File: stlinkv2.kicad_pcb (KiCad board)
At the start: 2 copper layers, 54 parts, among them J1 TX, J2 RX, J3 JTAG, J4 SWIMM, J5 USB_B, U1 AZ1117-3.3, U2 STM32F103C8Tx, Y1 8M

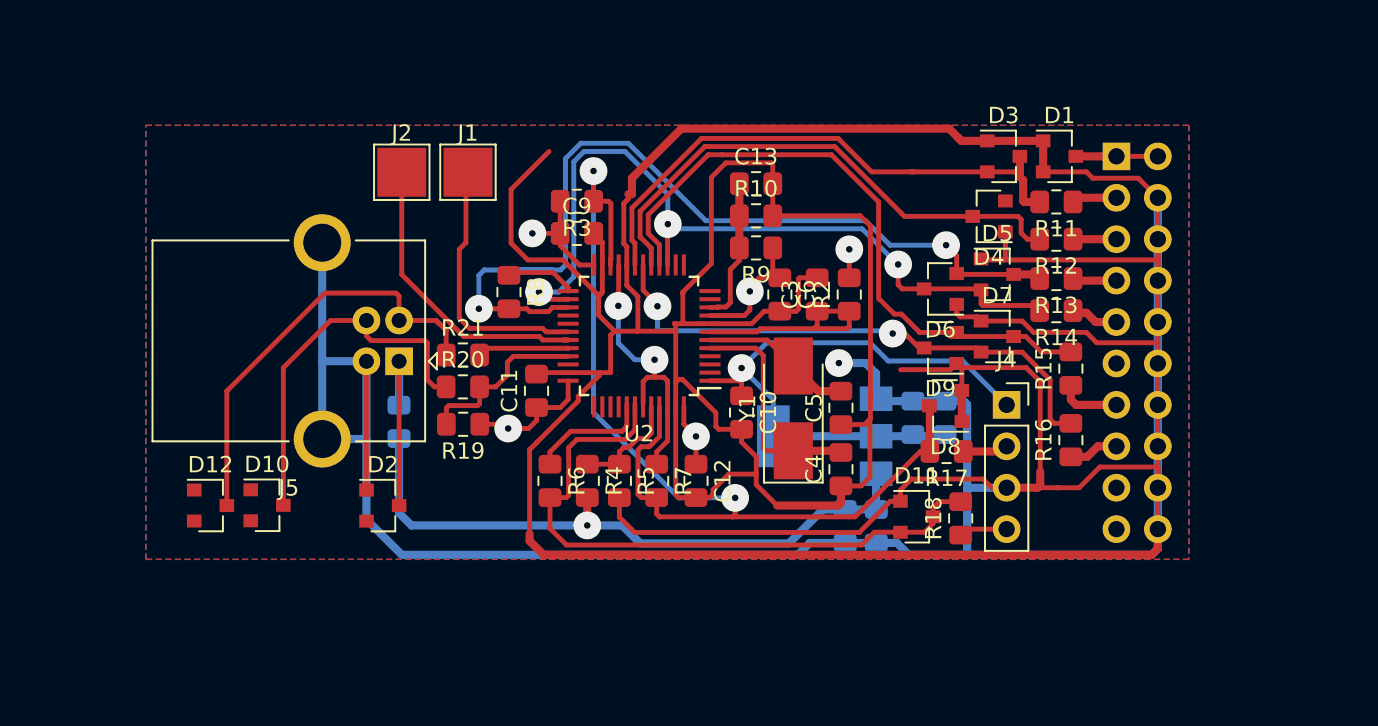
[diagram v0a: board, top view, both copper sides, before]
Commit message: добавил светодиоды, проверю без них
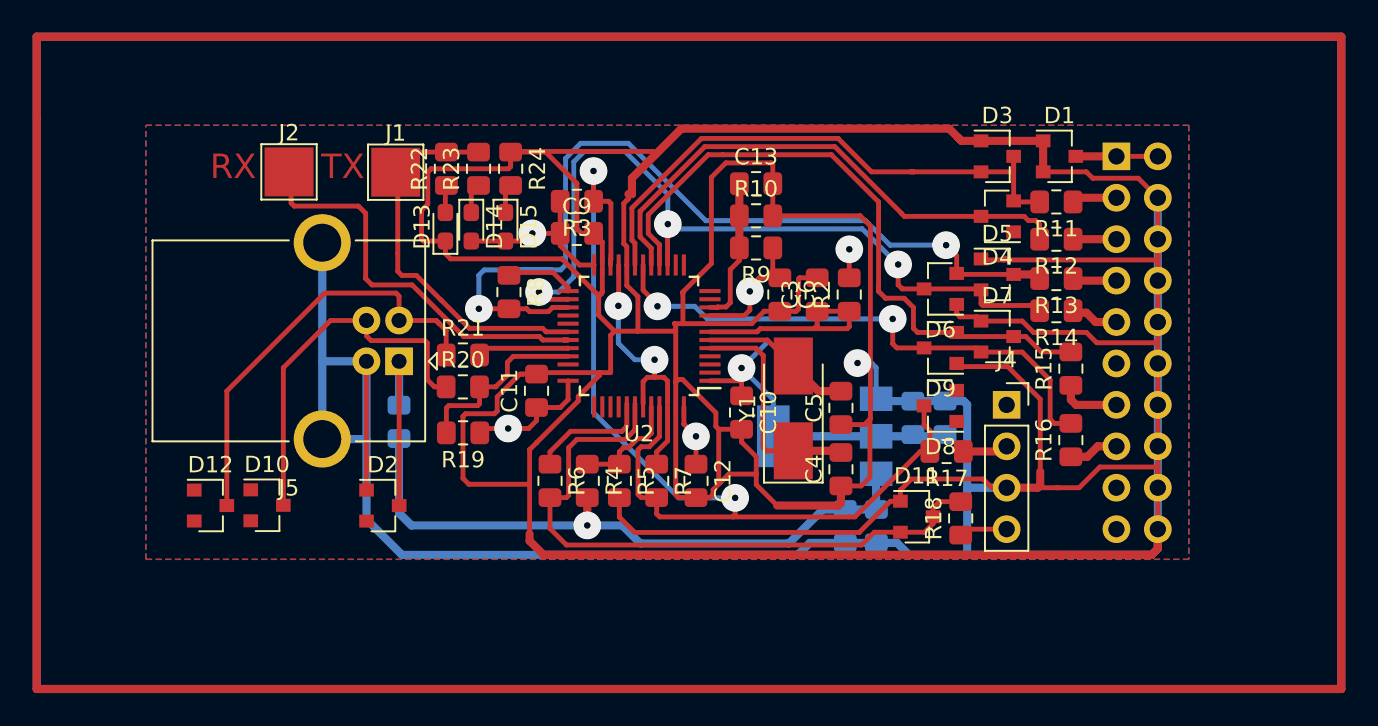
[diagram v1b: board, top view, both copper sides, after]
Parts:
- added D13: red, LED_SMD:LED_0603_1608Metric_Pad1.05x0.95mm_HandSolder, F.Cu at (115.1, 41.7)
- added D14: green, LED_SMD:LED_0603_1608Metric_Pad1.05x0.95mm_HandSolder, F.Cu at (116.6, 41.7)
- added D15: red, LED_SMD:LED_0603_1608Metric_Pad1.05x0.95mm_HandSolder, F.Cu at (118.7, 41.7)
- added R22: 100, Resistor_SMD:R_0805_2012Metric_Pad1.15x1.40mm_HandSolder, F.Cu at (115.1, 38.1)
- added R23: 100, Resistor_SMD:R_0805_2012Metric_Pad1.15x1.40mm_HandSolder, F.Cu at (117.1, 38.1)
- added R24: 100, Resistor_SMD:R_0805_2012Metric_Pad1.15x1.40mm_HandSolder, F.Cu at (119.1, 38.1)
- moved J2 6.91 mm to (105.5, 38.3)
- moved J1 4.43 mm to (112.0, 38.3)
- moved R19 0.53 mm to (116.1, 54.3)
- moved D4 0.51 mm to (148.9, 41.0)
- moved D3 0.38 mm to (148.9, 37.3)
- moved D8 0.32 mm to (145.4, 52.6)
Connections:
- net Net-(J1-Pad1) renamed /LED
- D1 pad : (no net) -> GND
- D11 pad : (no net) -> /SWIMM_RST
- D3 pad : (no net) -> /TRST
- D4 pad : (no net) -> /TRST
- D5 pad : (no net) -> /TCK_SWCLK
- D6 pad : (no net) -> /TMS_SWDIO
- D9 pad : (no net) -> /TDO_SWO
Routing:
- net (no net): track 0.00 -> 480.0 mm
- net GND: track 453.3 -> 488.9 mm
- net +3V3: track 73.8 -> 62.3 mm
- net /LED: track 16.3 -> 23.9 mm
- net Net-(J2-Pad1): track 18.4 -> 23.9 mm
- net Net-(D14-Pad1): track 0.00 -> 1.84 mm
- net Net-(D15-Pad1): track 0.00 -> 1.79 mm
- net Net-(D13-Pad2): track 0.00 -> 1.68 mm
- net /TRST: track 34.2 -> 35.4 mm
- net /NRST: track 33.6 -> 32.7 mm
- net /TDO_SWO: track 39.4 -> 40.2 mm
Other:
- board text added: "RX"
- board text added: "TX"
